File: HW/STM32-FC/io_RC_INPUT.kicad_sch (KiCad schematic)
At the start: 14 parts, among them J2 DSM, J4 RCIN, J5 SRXL2, J9 RSSI, Q1 S9013, U10 AMS1117-3.3

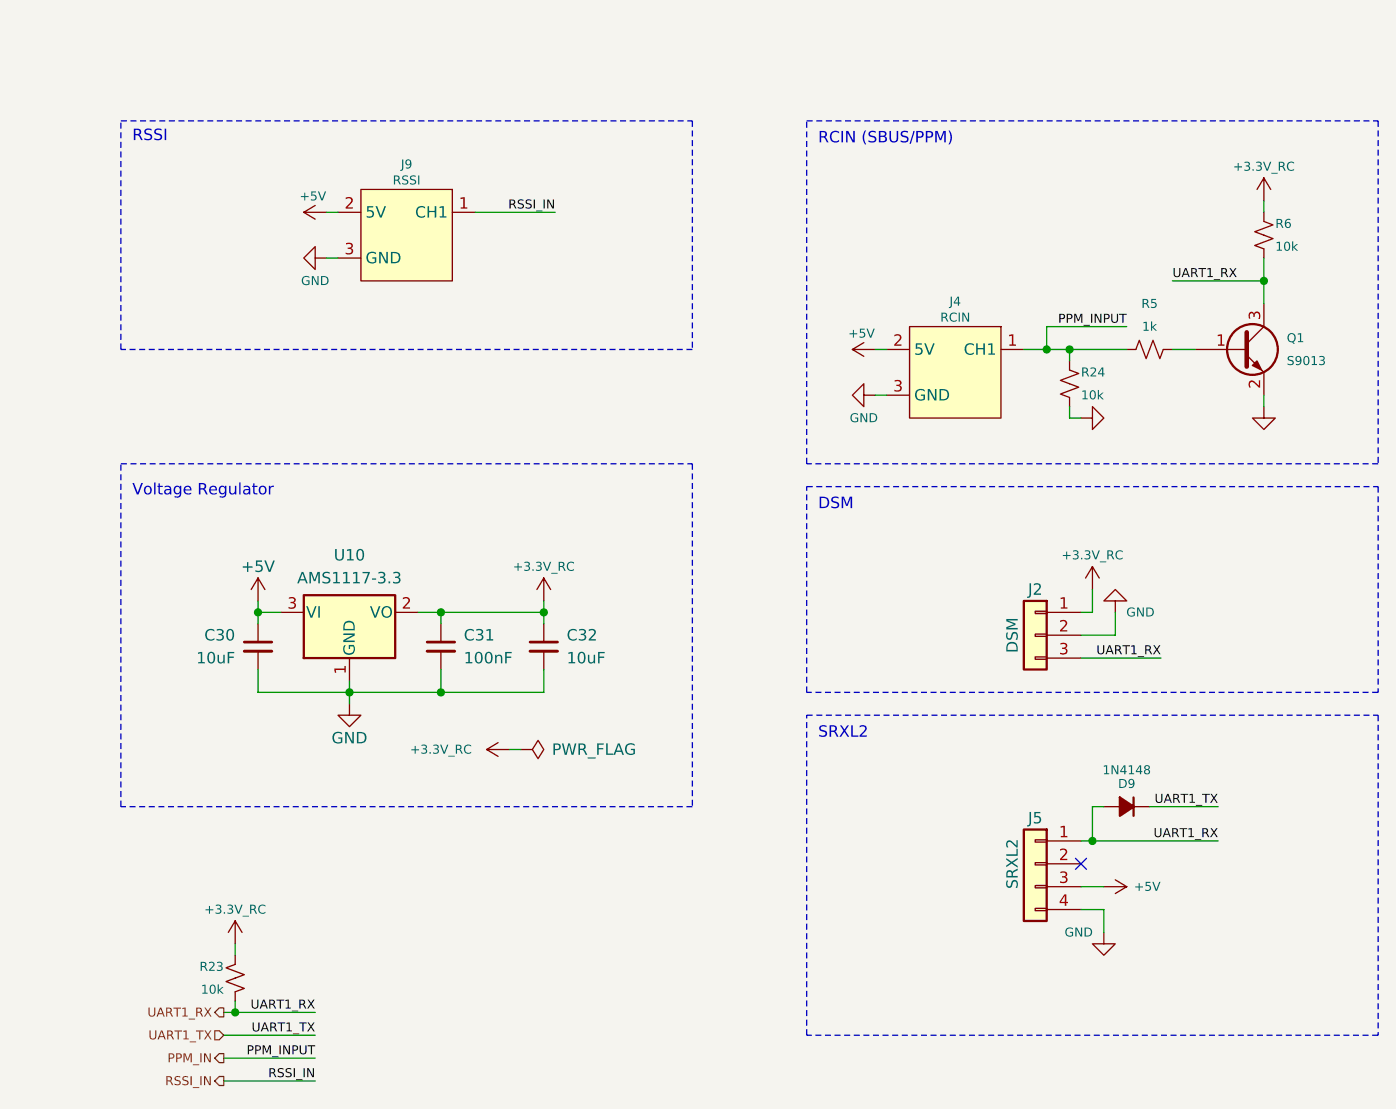
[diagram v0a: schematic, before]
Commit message: Big Update:IMU/RC/Conn./MCU
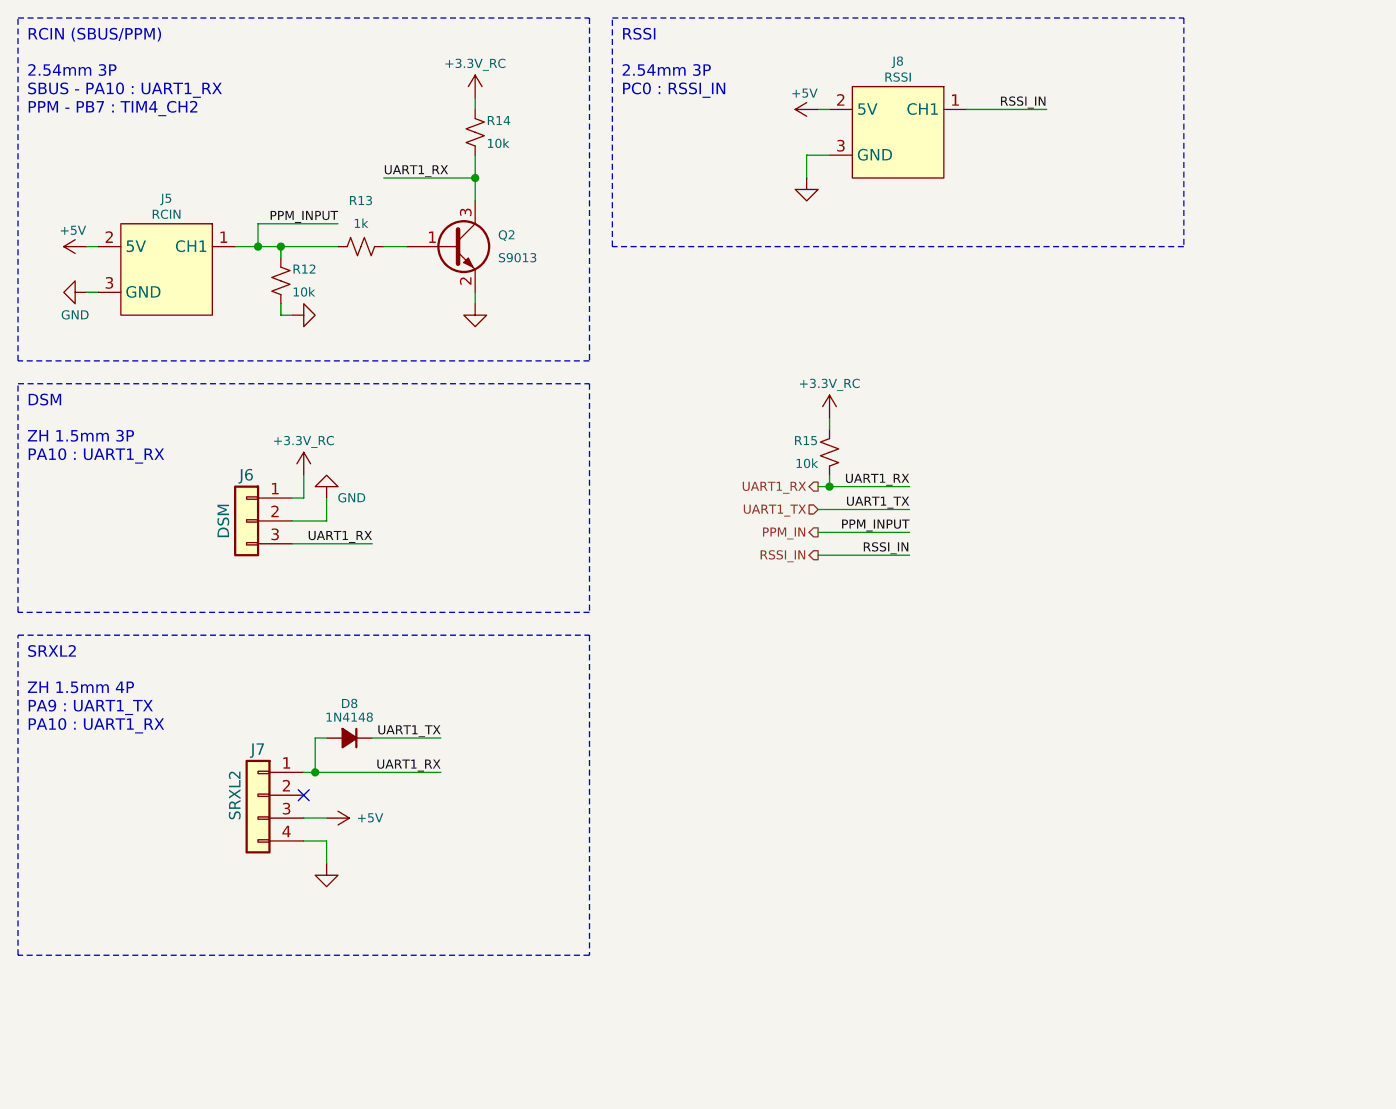
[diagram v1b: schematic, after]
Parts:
- removed C30, C32: 10uF, Capacitor_SMD:C_0402_1005Metric, symbol Device:C_Small
- removed C31: 100nF, Capacitor_SMD:C_0402_1005Metric, symbol Device:C_Small
- removed U10: AMS1117-3.3, Package_TO_SOT_SMD:SOT-223-3_TabPin2, symbol Regulator_Linear:AMS1117-3.3
- D8: renamed from D9; footprint (none) -> Diode_SMD:D_SOD-123
- J7: renamed from J5; footprint Connector_JST:JST_ZH_B3B-ZR-SM4-TF_1x03-1MP_P1.50mm_Vertical -> Connector_JST:JST_ZH_B4B-ZR-SM4-TF_1x04-1MP_P1.50mm_Vertical
- Q2: renamed from Q1; footprint digikey-footprints:SOT-23-3 -> Package_TO_SOT_SMD:SOT-23-3
- renumbered J4 to J5, J2 to J6, J9 to J8, R24 to R12, R5 to R13, R6 to R14, R23 to R15
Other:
- note added: "2.54mm 3P PC0 : RSSI_IN"
- note added: "2.54mm 3P SBUS - PA10 : UART1_RX PPM - PB7 : TIM4_CH2"
- note added: "ZH 1.5mm 3P PA10 : UART1_RX"
- note added: "ZH 1.5mm 4P PA9 : UART1_TX PA10 : UART1_RX"
- note removed: "Voltage Regulator"
- company: (none) -> INHA UNIV. NARAE
- title: (none) -> RC_INPUT
- moved on the sheet: D8, J5, J6, J7, J8, Q2, R12, R13, R14, R15
